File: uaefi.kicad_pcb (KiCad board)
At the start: 4 copper layers, 133.2 x 100 mm, 142 parts, among them J23 2-6447232-3, J25 2-6447232-3, J6 Conn_01x06, J7 Conn_01x05_Male, J8 USB_B_Mini, J9 USB_C, M1 Module-power_12and5V-0.3, M2 Module-knock-0.2, M3 Module-vr-discrete-0.5, M4 Module-vr-max9924-0.1, M5 Module-wbo-0.5, M6 Module:mega-mcu100/0.3, M7 Module-can-0.1, P1 Pad, P15 Pad, P16 Pad, P17 Pad, P18 Pad, P2 Pad, P3 Pad, P4 Pad, P5 Pad, P6 Pad, P7 Pad, P8 Pad, Q10 ISL9V3040D3ST, Q11 ISL9V3040D3ST, Q12 ISL9V3040D3ST, Q7 ISL9V3040D3ST, Q8 ISL9V3040D3ST, Q9 ISL9V3040D3ST, U1 TLE9201SG, U10 VNLD5160TR-E, U11 VNLD5160TR-E, U2 TLE9201SG, U3 MPX4/MPXH6400_MAP, U4 MAX31855KASA, U5 JDY-33, U6 VNLD5160TR-E, U7 VNLD5160TR-E, U8 VNLD5160TR-E, U9 VNLD5160TR-E

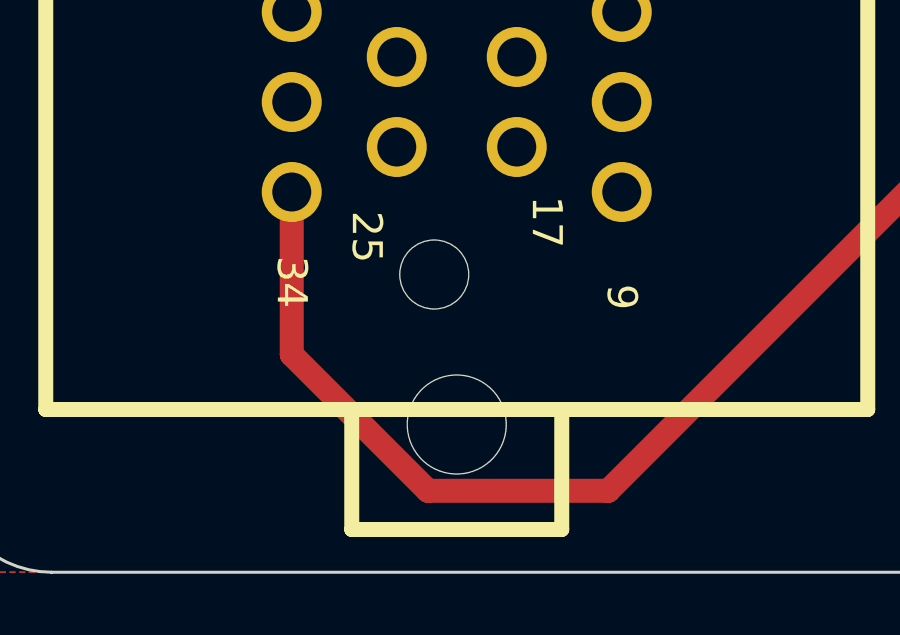
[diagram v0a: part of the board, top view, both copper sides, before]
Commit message: s
df
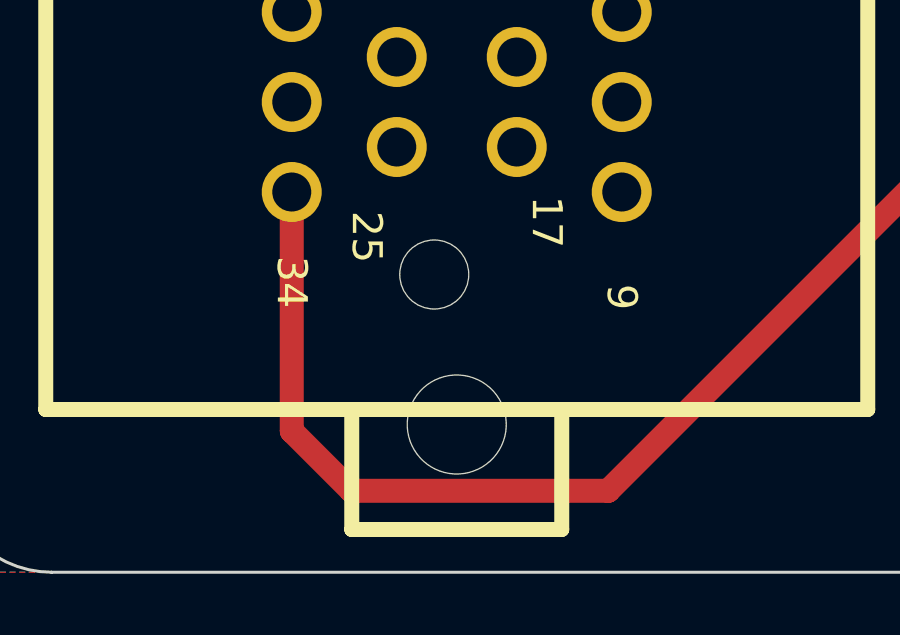
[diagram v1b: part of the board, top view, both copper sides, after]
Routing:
- net /OUT_DC1-: track 38.7 -> 40.2 mm
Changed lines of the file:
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@@
 	)
 	(segment
-		(start 38.874998 157.285)
-		(end 32.865 157.285)
+		(start 52.575001 144.095382)
+		(end 52.205381 144.465002)
+		(width 0.8)
+		(layer "F.Cu")
+		(net 4)
+	)
+	(segment
+		(start 51.149999 145.009999)
+		(end 38.874998 157.285)
+		(width 0.8)
+		(layer "F.Cu")
+		(net 4)
+	)
+	(segment
+		(start 52.575001 144)
+		(end 52.575001 144.095382)
+		(width 0.8)
+		(layer "F.Cu")
+		(net 4)
+	)
+	(segment
+		(start 28.325 155.295)
+		(end 28.325 147.325)
+		(width 0.8)
+		(layer "F.Cu")
+		(net 4)
+	)
+	(segment
+		(start 52.205381 144.465002)
+		(end 52.144997 144.465002)
+		(width 0.8)
+		(layer "F.Cu")
+		(net 4)
+	)
+	(segment
+		(start 30.315 157.285)
+		(end 28.325 155.295)
+		(width 0.8)
+		(layer "F.Cu")
+		(net 4)
+	)
+	(segment
+		(start 52.144997 144.465002)
+		(end 51.6 145.009999)
 		(width 0.8)
 		(layer "F.Cu")
@@
 	)
 	(segment
-		(start 52.575001 144.095382)
-		(end 52.205381 144.465002)
+		(start 38.874998 157.285)
+		(end 30.315 157.285)
 		(width 0.8)
 		(layer "F.Cu")
-		(net 4)
-	)
-	(segment
-		(start 52.575001 144)
-		(end 52.575001 144.095382)
-		(width 0.8)
-		(layer "F.Cu")
-		(net 4)
-	)
-	(segment
-		(start 51.149999 145.009999)
-		(end 38.874998 157.285)
-		(width 0.8)
-		(layer "F.Cu")
-		(net 4)
-	)
-	(segment
-		(start 32.865 157.285)
-		(end 28.325 152.745)
-		(width 0.8)
-		(layer "F.Cu")
-		(net 4)
-	)
-	(segment
-		(start 52.205381 144.465002)
-		(end 52.144997 144.465002)
-		(width 0.8)
-		(layer "F.Cu")
-		(net 4)
-	)
-	(segment
-		(start 52.144997 144.465002)
-		(end 51.6 145.009999)
-		(width 0.8)
-		(layer "F.Cu")
-		(net 4)
-	)
-	(segment
-		(start 28.325 152.745)
-		(end 28.325 147.325)
-		(width 0.8)
-		(layer "F.Cu")

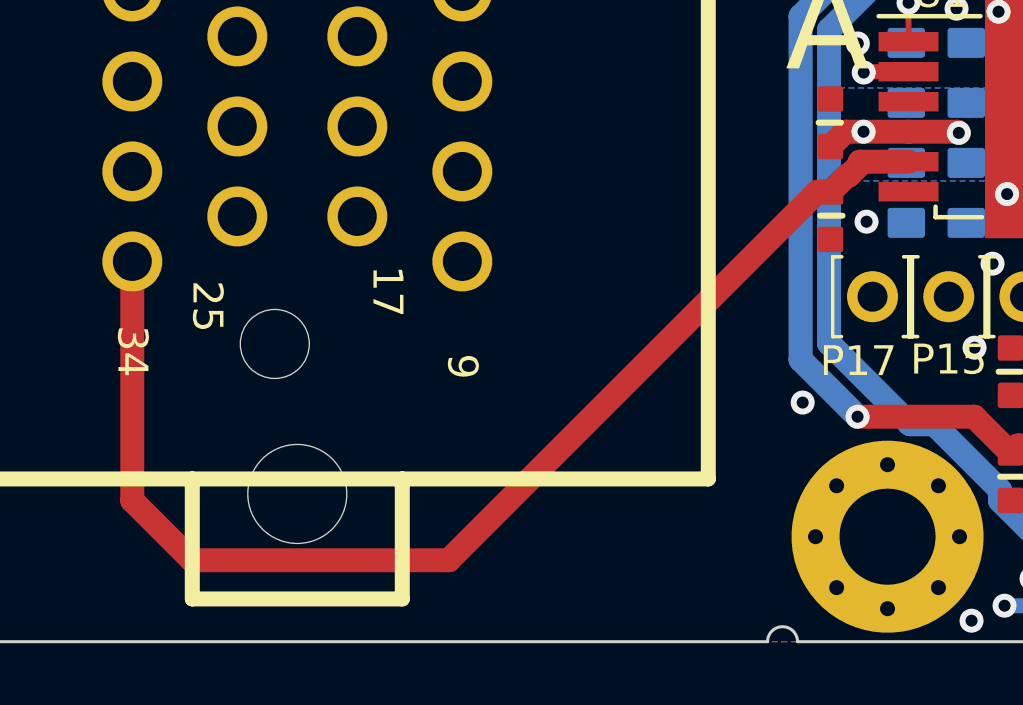
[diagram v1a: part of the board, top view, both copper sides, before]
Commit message: Update uaefi.kicad_pcb
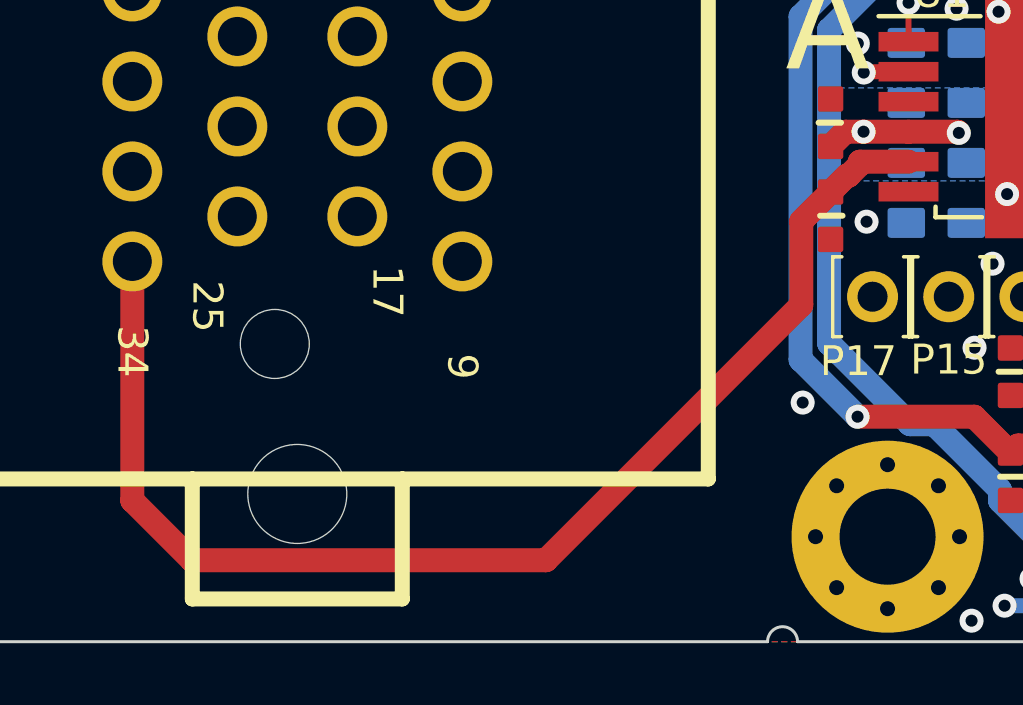
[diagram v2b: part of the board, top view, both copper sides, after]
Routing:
- net /OUT_DC1-: track 40.2 -> 41.9 mm
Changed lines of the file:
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@@
 	)
 	(segment
-		(start 52.575001 144.095382)
-		(end 52.205381 144.465002)
+		(start 28.325 155.295)
+		(end 28.325 147.325)
 		(width 0.8)
 		(layer "F.Cu")
@@
 	)
 	(segment
-		(start 51.149999 145.009999)
-		(end 38.874998 157.285)
+		(start 52.575001 144.095382)
+		(end 52.205381 144.465002)
 		(width 0.8)
 		(layer "F.Cu")
@@
 	)
 	(segment
-		(start 28.325 155.295)
-		(end 28.325 147.325)
+		(start 50.624999 145.985)
+		(end 50.624999 148.775001)
 		(width 0.8)
 		(layer "F.Cu")
@@
 	)
 	(segment
+		(start 52.144997 144.465002)
+		(end 51.6 145.009999)
+		(width 0.8)
+		(layer "F.Cu")
+		(net 4)
+	)
+	(segment
 		(start 30.315 157.285)
 		(end 28.325 155.295)
@@
 	)
 	(segment
-		(start 52.144997 144.465002)
-		(end 51.6 145.009999)
+		(start 51.6 145.009999)
+		(end 50.624999 145.985)
 		(width 0.8)
 		(layer "F.Cu")
@@
 	)
 	(segment
-		(start 51.6 145.009999)
-		(end 51.149999 145.009999)
+		(start 50.624999 148.775001)
+		(end 42.115 157.285)
 		(width 0.8)
 		(layer "F.Cu")
@@
 	)
 	(segment
-		(start 38.874998 157.285)
+		(start 42.115 157.285)
 		(end 30.315 157.285)
 		(width 0.8)

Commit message: AAa
AA
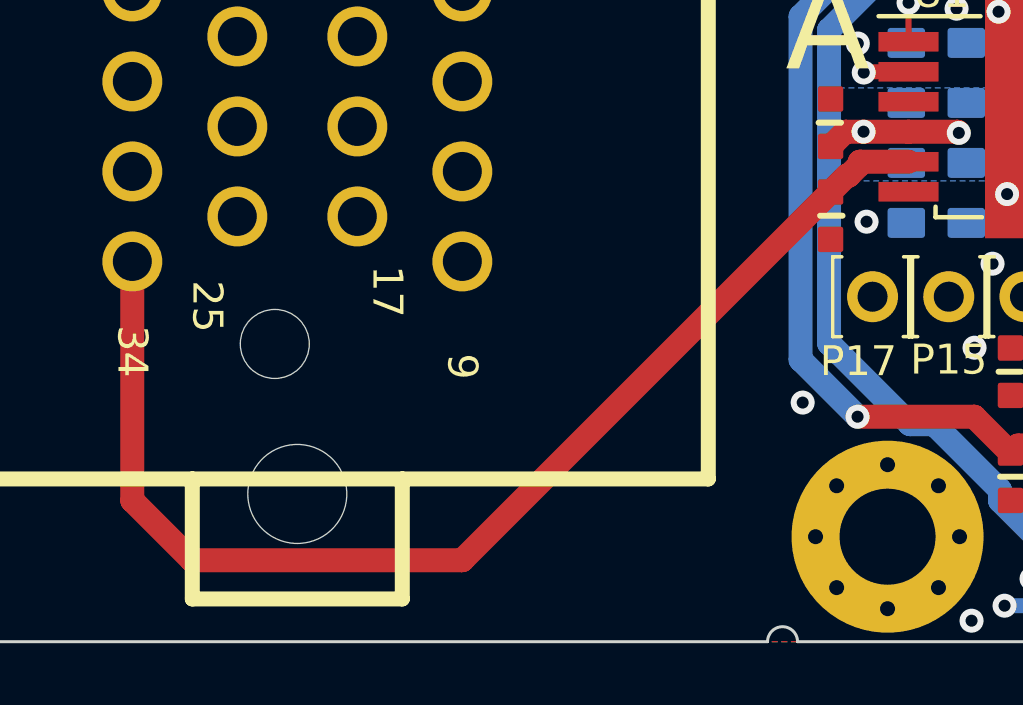
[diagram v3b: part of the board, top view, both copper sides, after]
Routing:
- net /OUT_DC1-: track 41.9 -> 40.2 mm
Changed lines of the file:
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@@
-	)
-	(segment
-		(start 28.325 155.295)
-		(end 28.325 147.325)
-		(width 0.8)
-		(layer "F.Cu")
-		(net 4)
 	)
 	(segment
@@
 	)
 	(segment
-		(start 50.624999 145.985)
-		(end 50.624999 148.775001)
+		(start 52.205381 144.465002)
+		(end 52.144997 144.465002)
 		(width 0.8)
 		(layer "F.Cu")
@@
 	)
 	(segment
-		(start 52.205381 144.465002)
-		(end 52.144997 144.465002)
+		(start 39.324999 157.285)
+		(end 30.315 157.285)
+		(width 0.8)
+		(layer "F.Cu")
+		(net 4)
+	)
+	(segment
+		(start 51.6 145.009999)
+		(end 39.324999 157.285)
 		(width 0.8)
 		(layer "F.Cu")
@@
 	)
 	(segment
-		(start 30.315 157.285)
-		(end 28.325 155.295)
+		(start 28.325 155.295)
+		(end 28.325 147.325)
 		(width 0.8)
 		(layer "F.Cu")
@@
 	)
 	(segment
-		(start 51.6 145.009999)
-		(end 50.624999 145.985)
+		(start 30.315 157.285)
+		(end 28.325 155.295)
 		(width 0.8)
 		(layer "F.Cu")
-		(net 4)
-	)
-	(segment
-		(start 50.624999 148.775001)
-		(end 42.115 157.285)
-		(width 0.8)
-		(layer "F.Cu")
-		(net 4)
-	)
-	(segment
-		(start 42.115 157.285)
-		(end 30.315 157.285)
-		(width 0.8)
-		(layer "F.Cu")
